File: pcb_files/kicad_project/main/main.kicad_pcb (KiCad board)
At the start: 2 copper layers, 100 x 71.3 mm, 155 parts, among them IC1 AS5145B-HSST, IC2 AS5145B-HSST, J1 Conn_01x02_Socket, J2 Conn_01x04_Socket, Q1 AON7423, Y1 Crystal_GND24

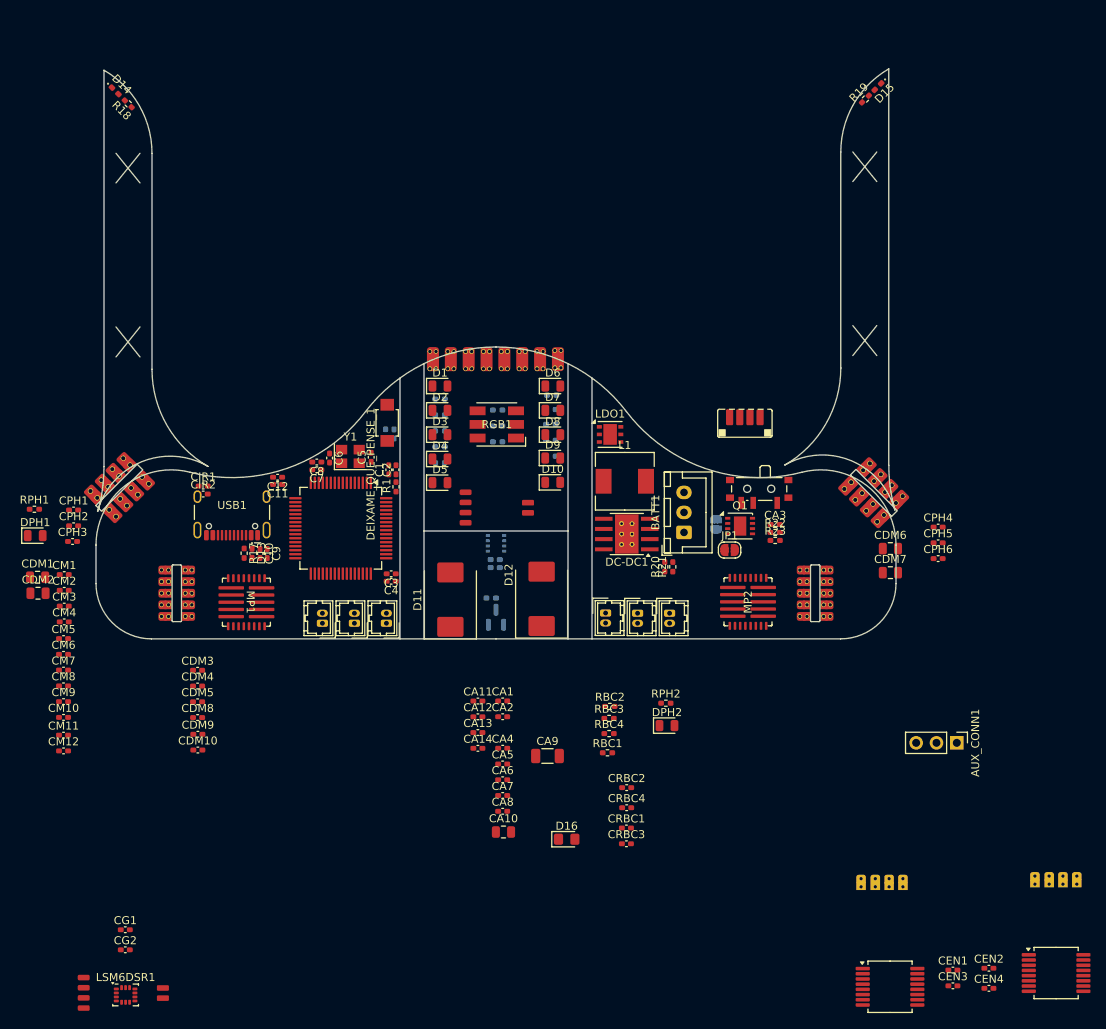
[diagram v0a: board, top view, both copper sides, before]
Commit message: "Finaliza" (CREO) la PCB main de DragonBot2
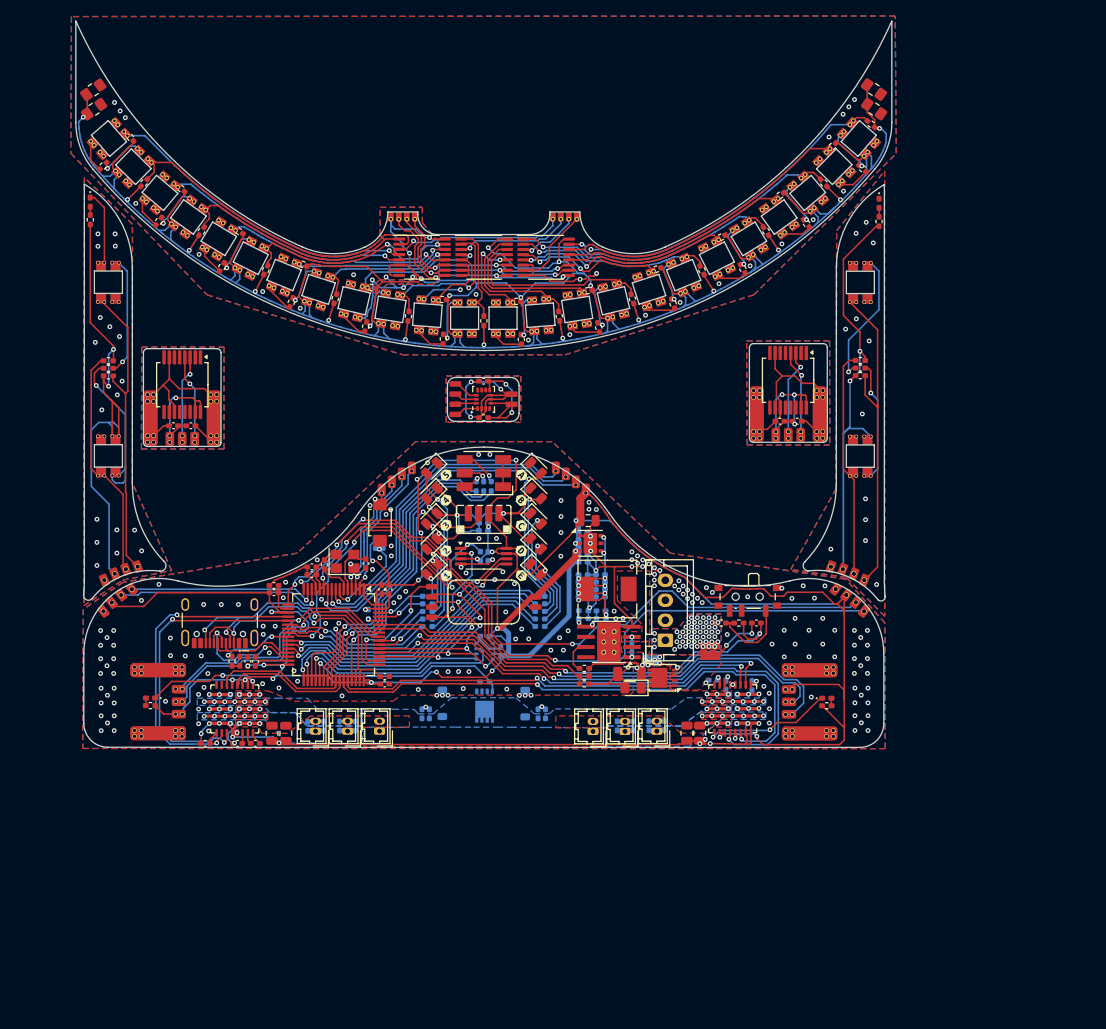
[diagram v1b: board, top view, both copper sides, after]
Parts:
- removed AUX_CONN1: Conn_01x03_Pin, Connector_PinHeader_2.54mm:PinHeader_1x03_P2.54mm_Vertical
- added C13: 10uF, Capacitor_SMD:C_0805_2012Metric_Pad1.18x1.45mm_HandSolder, F.Cu at (193.2, 49.4)
- added C15: 0.1uF, Capacitor_SMD:C_0805_2012Metric_Pad1.18x1.45mm_HandSolder, F.Cu at (95.7, 49.4)
- added C17: 10uF, Capacitor_SMD:C_0805_2012Metric_Pad1.18x1.45mm_HandSolder, F.Cu at (193.1, 46.9)
- added C18: 0.1uF, Capacitor_SMD:C_0805_2012Metric_Pad1.18x1.45mm_HandSolder, F.Cu at (95.6, 47.0)
- added CONN_MORRO1: Conn_01x08_Pin, custom_footprints:DragonBot_pads_morro, F.Cu at (144.4, 63.1)
- added CSRAM1: 0.1uF, Capacitor_SMD:C_0402_1005Metric_Pad0.74x0.62mm_HandSolder, B.Cu at (144.9, 105.3)
- added MUX1: CD4051B, custom_footprints:MUX_CD4051B, F.Cu at (152.2, 67.9)
- added MUX2: CD4051B, custom_footprints:MUX_CD4051B, F.Cu at (144.4, 67.9)
- added MUX3: CD4051B, custom_footprints:MUX_CD4051B, F.Cu at (136.7, 67.9)
- added R24: 10k, Resistor_SMD:R_0402_1005Metric_Pad0.72x0.64mm_HandSolder, F.Cu at (97.4, 80.8)
- added R25: 1K, Resistor_SMD:R_0402_1005Metric_Pad0.72x0.64mm_HandSolder, F.Cu at (95.2, 63.2)
- added R26: 45, Resistor_SMD:R_0402_1005Metric_Pad0.72x0.64mm_HandSolder, F.Cu at (191.4, 81.8)
- added R27: 10k, Resistor_SMD:R_0402_1005Metric_Pad0.72x0.64mm_HandSolder, F.Cu at (191.4, 82.7)
- added R28: 45, Resistor_SMD:R_0402_1005Metric_Pad0.72x0.64mm_HandSolder, F.Cu at (97.4, 81.8)
- added R29: 10k, Resistor_SMD:R_0402_1005Metric_Pad0.72x0.64mm_HandSolder, F.Cu at (97.4, 82.7)
- added R30: 45, Resistor_SMD:R_0402_1005Metric_Pad0.72x0.64mm_HandSolder, F.Cu at (191.7, 56.8)
- added R31: 10k, Resistor_SMD:R_0402_1005Metric_Pad0.72x0.64mm_HandSolder, F.Cu at (192.8, 51.3)
- added R32: 10k, Resistor_SMD:R_0402_1005Metric_Pad0.72x0.64mm_HandSolder, F.Cu at (188.0, 54.0)
- added R33: 45, Resistor_SMD:R_0402_1005Metric_Pad0.72x0.64mm_HandSolder, F.Cu at (184.7, 63.7)
- added R34: 10k, Resistor_SMD:R_0402_1005Metric_Pad0.72x0.64mm_HandSolder, F.Cu at (186.9, 58.6)
- added R35: 10k, Resistor_SMD:R_0402_1005Metric_Pad0.72x0.64mm_HandSolder, F.Cu at (181.4, 60.2)
- added R36: 45, Resistor_SMD:R_0402_1005Metric_Pad0.72x0.64mm_HandSolder, F.Cu at (176.8, 69.3)
- added R37: 10k, Resistor_SMD:R_0402_1005Metric_Pad0.72x0.64mm_HandSolder, F.Cu at (179.7, 64.6)
- added R38: 10k, Resistor_SMD:R_0402_1005Metric_Pad0.72x0.64mm_HandSolder, F.Cu at (174.0, 65.4)
- added R39: 45, Resistor_SMD:R_0402_1005Metric_Pad0.72x0.64mm_HandSolder, F.Cu at (168.0, 73.7)
- added R40: 10k, Resistor_SMD:R_0402_1005Metric_Pad0.72x0.64mm_HandSolder, F.Cu at (171.7, 69.5)
- added R41: 10k, Resistor_SMD:R_0402_1005Metric_Pad0.72x0.64mm_HandSolder, F.Cu at (166.0, 69.4)
- added R42: 45, Resistor_SMD:R_0402_1005Metric_Pad0.72x0.64mm_HandSolder, F.Cu at (158.7, 76.7)
- added R43: 10k, Resistor_SMD:R_0402_1005Metric_Pad0.72x0.64mm_HandSolder, F.Cu at (163.0, 73.1)
- added R44: 10k, Resistor_SMD:R_0402_1005Metric_Pad0.72x0.64mm_HandSolder, F.Cu at (157.3, 72.1)
- added R45: 45, Resistor_SMD:R_0402_1005Metric_Pad0.72x0.64mm_HandSolder, F.Cu at (149.1, 78.2)
- added R46: 10k, Resistor_SMD:R_0402_1005Metric_Pad0.72x0.64mm_HandSolder, F.Cu at (153.8, 75.3)
- added R47: 10k, Resistor_SMD:R_0402_1005Metric_Pad0.72x0.64mm_HandSolder, F.Cu at (148.4, 73.4)
- added R48: 45, Resistor_SMD:R_0402_1005Metric_Pad0.72x0.64mm_HandSolder, F.Cu at (139.3, 78.1)
- added R49: 10k, Resistor_SMD:R_0402_1005Metric_Pad0.72x0.64mm_HandSolder, F.Cu at (144.4, 75.9)
- added R50: 10k, Resistor_SMD:R_0402_1005Metric_Pad0.72x0.64mm_HandSolder, F.Cu at (139.1, 73.2)
- added R51: 45, Resistor_SMD:R_0402_1005Metric_Pad0.72x0.64mm_HandSolder, F.Cu at (129.6, 76.6)
- added R52: 10k, Resistor_SMD:R_0402_1005Metric_Pad0.72x0.64mm_HandSolder, F.Cu at (135.0, 75.3)
- added R53: 10k, Resistor_SMD:R_0402_1005Metric_Pad0.72x0.64mm_HandSolder, F.Cu at (130.3, 71.7)
- added R54: 45, Resistor_SMD:R_0402_1005Metric_Pad0.72x0.64mm_HandSolder, F.Cu at (120.3, 73.5)
- added R55: 10k, Resistor_SMD:R_0402_1005Metric_Pad0.72x0.64mm_HandSolder, F.Cu at (125.8, 73.1)
- added R56: 10k, Resistor_SMD:R_0402_1005Metric_Pad0.72x0.64mm_HandSolder, F.Cu at (121.7, 68.8)
- added R57: 45, Resistor_SMD:R_0402_1005Metric_Pad0.72x0.64mm_HandSolder, F.Cu at (111.6, 69.1)
- added R58: 10k, Resistor_SMD:R_0402_1005Metric_Pad0.72x0.64mm_HandSolder, F.Cu at (117.1, 69.5)
- added R59: 10k, Resistor_SMD:R_0402_1005Metric_Pad0.72x0.64mm_HandSolder, F.Cu at (113.7, 64.6)
- added R60: 45, Resistor_SMD:R_0402_1005Metric_Pad0.72x0.64mm_HandSolder, F.Cu at (103.7, 63.4)
- added R61: 10k, Resistor_SMD:R_0402_1005Metric_Pad0.72x0.64mm_HandSolder, F.Cu at (109.1, 64.7)
- added R62: 10k, Resistor_SMD:R_0402_1005Metric_Pad0.72x0.64mm_HandSolder, F.Cu at (106.5, 59.3)
- added R63: 45, Resistor_SMD:R_0402_1005Metric_Pad0.72x0.64mm_HandSolder, F.Cu at (96.8, 56.5)
- added R64: 10k, Resistor_SMD:R_0402_1005Metric_Pad0.72x0.64mm_HandSolder, F.Cu at (101.9, 58.6)
- added R65: 10k, Resistor_SMD:R_0402_1005Metric_Pad0.72x0.64mm_HandSolder, F.Cu at (100.2, 52.9)
- added RRAM1: 10K, Resistor_SMD:R_0402_1005Metric_Pad0.72x0.64mm_HandSolder, B.Cu at (143.9, 105.3)
- added S1: ~, custom_footprints:DragonBot2_QRE1113, F.Cu at (191.2, 53.1)
- added S10: ~, custom_footprints:DragonBot2_QRE1113, F.Cu at (156.0, 74.4)
- added S11: ~, custom_footprints:DragonBot2_QRE1113, F.Cu at (151.4, 75.1)
- added S12: ~, custom_footprints:DragonBot2_QRE1113, F.Cu at (146.8, 75.5)
- added S13: ~, custom_footprints:DragonBot2_QRE1113, F.Cu at (142.0, 75.5)
- added S14: ~, custom_footprints:DragonBot2_QRE1113, F.Cu at (137.3, 75.1)
- added S15: ~, custom_footprints:DragonBot2_QRE1113, F.Cu at (132.7, 74.4)
- added S16: ~, custom_footprints:DragonBot2_QRE1113, F.Cu at (128.2, 73.3)
- added S17: ~, custom_footprints:DragonBot2_QRE1113, F.Cu at (123.7, 71.9)
- added S18: ~, custom_footprints:DragonBot2_QRE1113, F.Cu at (119.4, 70.1)
- added S19: ~, custom_footprints:DragonBot2_QRE1113, F.Cu at (115.2, 68.0)
- added S2: ~, custom_footprints:DragonBot2_QRE1113, F.Cu at (188.2, 56.6)
- added S20: ~, custom_footprints:DragonBot2_QRE1113, F.Cu at (111.3, 65.6)
- added S21: ~, custom_footprints:DragonBot2_QRE1113, F.Cu at (107.5, 62.9)
- added S22: ~, custom_footprints:DragonBot2_QRE1113, F.Cu at (103.9, 59.9)
- added S23: ~, custom_footprints:DragonBot2_QRE1113, F.Cu at (100.6, 56.6)
- added S24: ~, custom_footprints:DragonBot2_QRE1113, F.Cu at (97.5, 53.1)
- added S3: ~, custom_footprints:DragonBot2_QRE1113, F.Cu at (184.9, 59.9)
- added S4: ~, custom_footprints:DragonBot2_QRE1113, F.Cu at (181.3, 62.9)
- added S5: ~, custom_footprints:DragonBot2_QRE1113, F.Cu at (177.5, 65.6)
- added S6: ~, custom_footprints:DragonBot2_QRE1113, F.Cu at (173.5, 68.0)
- added S7: ~, custom_footprints:DragonBot2_QRE1113, F.Cu at (169.4, 70.1)
- added S8: ~, custom_footprints:DragonBot2_QRE1113, F.Cu at (165.0, 71.9)
- added S9: ~, custom_footprints:DragonBot2_QRE1113, F.Cu at (160.6, 73.3)
- added SEN_MARK_CONN_L1: Conn_01x04_Socket, custom_footprints:DragonBot_pad_marcas, F.Cu at (189.9, 107.4)
- added SEN_MARK_CONN_R1: Conn_01x04_Socket, custom_footprints:DragonBot_pad_marcas, F.Cu at (99.0, 107.4)
- added SML1: ~, custom_footprints:FujitoraBot2_QRE1113, F.Cu at (191.4, 92.8)
- added SML2: ~, custom_footprints:FujitoraBot2_QRE1113, F.Cu at (191.4, 71.1)
- added SMR1: ~, custom_footprints:FujitoraBot2_QRE1113, F.Cu at (97.4, 92.7)
- added SMR2: ~, custom_footprints:FujitoraBot2_QRE1113, F.Cu at (97.4, 71.0)
- added SRAM1: 23AA04M-I/ST, Package_SO:TSSOP-8_4.4x3mm_P0.65mm, F.Cu at (144.4, 105.3)
- added kibuzzard-696C1621: G***, kibuzzard-696C1621, F.Cu at (139.7, 107.7)
- added kibuzzard-696C163C: G***, kibuzzard-696C163C, F.Cu at (139.6, 104.6)
- added kibuzzard-696C164F: G***, kibuzzard-696C164F, F.Cu at (139.6, 101.4)
- added kibuzzard-696C1681: G***, kibuzzard-696C1681, F.Cu at (139.7, 98.3)
- added kibuzzard-696C1693: G***, kibuzzard-696C1693, F.Cu at (139.7, 95.1)
- added kibuzzard-696C16A9: G***, kibuzzard-696C16A9, F.Cu at (149.1, 95.1)
- added kibuzzard-696C16F5: G***, kibuzzard-696C16F5, F.Cu at (149.1, 98.3)
- added kibuzzard-696C171C: G***, kibuzzard-696C171C, F.Cu at (149.1, 101.5)
- added kibuzzard-696C172A: G***, kibuzzard-696C172A, F.Cu at (149.1, 104.6)
- added kibuzzard-696C173B: G***, kibuzzard-696C173B, F.Cu at (149.1, 107.7)
- ARRAY_MORRO1: footprint custom_footprints:Fujitora_pads_morro -> custom_footprints:DragonBot_pads_main
- BATT1: value Conn_01x03_Pin -> Conn_01x04_Socket; footprint Connector_JST:JST_XH_B3B-XH-A_1x03_P2.50mm_Vertical -> Connector_JST:JST_XH_B4B-XH-AM_1x04_P2.50mm_Vertical
- BUK9Q20-40H1: footprint Package_TO_SOT_SMD:SOT-23 -> custom_footprints:Mosfet_succion_BUK9Q20
- CA1, CA11, CA12, CA13, CA14, CA2, CA4, CA5, CA6, CA7, CA8, CDM10, CDM3, CDM4, CDM5, CDM8, CDM9, CIR1, CIR2, CM1, CM10, CM11, CM12, CM2, CM3, CM4, CM5, CM6, CM7, CM8, CM9, CPH4, CPH5, CPH6, CRBC1, CRBC2, CRBC3, CRBC4, R1, RBC1, RBC3, RBC4: moved to B.Cu
- CONN_ENC_L1, CONN_ENC_R1: footprint custom_footprints:FujitoraBot2_PCBmodule_encoder -> custom_footprints:DragonBot2_Encoder_main
- D11, D12: value B340 -> SS34FA; footprint Diode_SMD:D_SMC -> Diode_SMD:D_SOD-123; moved to B.Cu
- DPH1, DPH2: footprint LED_SMD:LED_0805_2012Metric -> LED_SMD:LED_0402_1005Metric_Pad0.77x0.64mm_HandSolder
- ENC_L1, ENC_R1: footprint custom_footprints:ZoroBot3_PCBmain_Encoder -> custom_footprints:DragonBot2_Encoder_main
- Q1: footprint Package_DFN_QFN:DFN-8-1EP_3x3mm_P0.65mm_EP1.55x2.4mm -> custom_footprints:AON7423
- R19: value 1K -> 10k
- SEN_MARK_L1, SEN_MARK_R1: footprint custom_footprints:ZoroBot3_Main_sensors -> custom_footprints:DragonBot_pad_marcas
- moved IC2 131.7 mm to (106.7, 83.8), turned to -90 degrees
- moved CEN4 123.8 mm to (105.6, 89.0), turned to 180 degrees
- moved CONN_ENC_R1 122.2 mm to (106.7, 91.1), turned to 90 degrees
- moved CEN3 118.2 mm to (107.8, 89.0)
- moved D15 99.5 mm to (95.2, 61.0), turned to -90 degrees
- moved D14 96.5 mm to (193.8, 61.2), turned to -90 degrees
- moved R18 95.0 mm to (193.8, 63.4), turned to 90 degrees
- moved J2 87.6 mm to (140.8, 85.7)
- moved LSM6DSR1 86.9 mm to (144.3, 85.7), turned to 90 degrees
- moved J1 86.1 mm to (147.8, 85.7), turned to 180 degrees
- moved CG2 84.0 mm to (144.3, 83.4), turned to 180 degrees
- moved ENC_L1 80.3 mm to (106.7, 123.5), turned to 180 degrees
- moved CG1 78.1 mm to (144.3, 88.0), turned to 180 degrees
- moved ENC_R1 77.3 mm to (182.1, 123.5)
- moved IC1 76.9 mm to (182.4, 83.3), turned to -90 degrees
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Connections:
- BATT1 pad 3: GND -> unconnected-(BATT1-Pin_3-Pad3)
- BUK9Q20-40H1 pad 1: /MOT_S- -> GND
- BUK9Q20-40H1 pad 2: /PWM_SUCC -> GND
- CM1 pad 1: GND -> /MOT_L-
- CM1 pad 2: /BATT -> /MOT_L+
- CM10 pad 1: GND -> /MOT_S-
- CM11 pad 1: GND -> /MOT_S-
- CM12 pad 1: GND -> /MOT_S-
- CM2 pad 1: GND -> /MOT_L-
- CM2 pad 2: /BATT -> /MOT_L+
- CM3 pad 1: GND -> /MOT_L-
- CM3 pad 2: /BATT -> /MOT_L+
- CM4 pad 1: GND -> /MOT_L-
- CM4 pad 2: /BATT -> /MOT_L+
- CM5 pad 1: GND -> /MOT_R-
- CM5 pad 2: /BATT -> /MOT_R+
- CM6 pad 1: GND -> /MOT_R-
- CM6 pad 2: /BATT -> /MOT_R+
- CM7 pad 1: GND -> /MOT_R-
- CM7 pad 2: /BATT -> /MOT_R+
- CM8 pad 1: GND -> /MOT_R-
- CM8 pad 2: /BATT -> /MOT_R+
- CM9 pad 1: GND -> /MOT_S-
- D14 pad 1: GND -> /Sensores/GND_ML
- D15 pad 1: GND -> /Sensores/GND_MR
- DEIXAME_QUE_PENSE_1 pad 2: /OUT_MUX_A -> /OUT_MUX_C
- DEIXAME_QUE_PENSE_1 pad 24: /AUX_PIN -> /NSS_SRAM
- DEIXAME_QUE_PENSE_1 pad 26: /LED8 -> /LED6
- DEIXAME_QUE_PENSE_1 pad 27: /LED9 -> /LED7
- DEIXAME_QUE_PENSE_1 pad 28: /LED10 -> /LED8
- DEIXAME_QUE_PENSE_1 pad 33: /LED7 -> /LED9
- DEIXAME_QUE_PENSE_1 pad 34: /LED6 -> /LED10
- DEIXAME_QUE_PENSE_1 pad 4: /OUT_MUX_C -> /OUT_MUX_A
- DEIXAME_QUE_PENSE_1 pad 41: /PWM_MOT_RB -> /PWM_MOT_LB
- DEIXAME_QUE_PENSE_1 pad 42: /PWM_MOT_RA -> /PWM_MOT_LA
- DEIXAME_QUE_PENSE_1 pad 43: /PWM_MOT_LB -> /PWM_MOT_RB
- DEIXAME_QUE_PENSE_1 pad 44: /PWM_MOT_LA -> /PWM_MOT_RA
- DEIXAME_QUE_PENSE_1 pad 56: /ENC_R_B -> /ENC_L_A
- DEIXAME_QUE_PENSE_1 pad 57: /ENC_R_A -> /ENC_L_B
- DEIXAME_QUE_PENSE_1 pad 58: /ENC_L_B -> /ENC_R_A
- DEIXAME_QUE_PENSE_1 pad 59: /ENC_L_A -> /ENC_R_B
- JP2 pad 1: /BATT -> Net-(JP1-A)
- JP2 pad 2: Net-(JP1-A) -> /BATT
- MP2 pad 10: /MOT_R- -> /MOT_R+
- MP2 pad 12: /MOT_R+ -> /MOT_R-
- MP2 pad 23: /MOT_R+ -> /MOT_R-
- MP2 pad 25: /MOT_R- -> /MOT_R+
- Q1 pad 1: /BATT -> Net-(JP1-A)
- Q1 pad 2: Net-(Q1-G) -> Net-(JP1-A)
- Q1 pad 4: (no net) -> Net-(Q1-G)
- Q1 pad 5: (no net) -> /BATT
- Q1 pad 6: (no net) -> /BATT
- Q1 pad 7: (no net) -> /BATT
- Q1 pad 8: (no net) -> /BATT
- R18 pad 1: +3V3 -> /Sensores/3.3_ML
- R19 pad 1: +3V3 -> /Sensores/MARK_L1
- R19 pad 2: Net-(D15-A) -> /Sensores/3.3_ML
- USB1 pad 11: +3V3 -> unconnected-(USB1-VBUS-Pad11)
- USB1 pad 2: +3V3 -> unconnected-(USB1-VBUS-Pad2)
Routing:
- net +3V3: track 0.00 -> 406.8 mm, vias 0 -> 25
- net /Sensores/3.3_M: track 0.00 -> 354.9 mm, vias 0 -> 21
- net GND: track 0.00 -> 223.3 mm, vias 0 -> 205
- net /IN_MARK_R2: track 0.00 -> 91.8 mm, vias 0 -> 3
- net /IN_MARK_R1: track 0.00 -> 87.2 mm, vias 0 -> 3
- net /PWM_MOT_RA: track 0.00 -> 71.6 mm, vias 0 -> 2
- net /PWM_MOT_RB: track 0.00 -> 69.0 mm, vias 0 -> 2
- net /IN_CURR_MR_A: track 0.00 -> 66.1 mm, vias 0 -> 4
- net /Sensores/3.3_MR: track 0.00 -> 64.0 mm, vias 0 -> 2
- net /IN_CURR_MR_B: track 0.00 -> 64.0 mm, vias 0 -> 4
- net /ENC_R_B: track 0.00 -> 62.2 mm, vias 0 -> 1
- net /ENC_R_A: track 0.00 -> 59.9 mm, vias 0 -> 1
- net /Sensores/3.3_ML: track 0.00 -> 53.1 mm, vias 0 -> 2
- net /Sensores/GND_M: track 0.00 -> 52.4 mm, vias 0 -> 29
- net /BATT_VOLTAGE: track 0.00 -> 47.7 mm, vias 0 -> 2
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- added copper zone on F.Cu, net /BATT
- added copper zone on B.Cu, net /ENC_L_GND
- added copper zone on F.Cu, net /ENC_L_GND
- added copper zone on B.Cu, net /ENC_R_GND
- added copper zone on F.Cu, net /ENC_R_GND
- added copper zone on B.Cu, net /GND_MPU
- added copper zone on F.Cu, net /GND_MPU
- added copper zone on B.Cu, net /LIPO+
- added copper zone on F.Cu, net /LIPO+
- added copper zone on B.Cu, net /MOT_L+
- added copper zone on B.Cu, net /MOT_L-
- added copper zone on B.Cu, net /MOT_R+
- added copper zone on B.Cu, net /MOT_R-
- added copper zone on B.Cu, net /MOT_S-
- added copper zone on B.Cu, net /Sensores/3.3_M
- added copper zone on F.Cu, net /Sensores/3.3_M
- added copper zone on B.Cu, net /Sensores/GND_M
- added copper zone on F.Cu, net /Sensores/GND_M
- added copper zone on B.Cu, net /Sensores/GND_ML
- added copper zone on F.Cu, net /Sensores/GND_ML
- added copper zone on B.Cu, net /Sensores/GND_MR
- added copper zone on F.Cu, net /Sensores/GND_MR
- added copper zone on B.Cu, net GND
- added copper zone on F.Cu, net GND
- added copper zone on F.Cu, net Net-(DC-DC1-SW)
- added copper zone on F.Cu, net Net-(JP1-A)
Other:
- board size 100 x 71.3 mm -> 102 x 90.8 mm
